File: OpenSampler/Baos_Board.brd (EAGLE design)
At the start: 57.2 x 26 mm, 33 parts, among them U1 FRAM, U2 DS3231ST&R

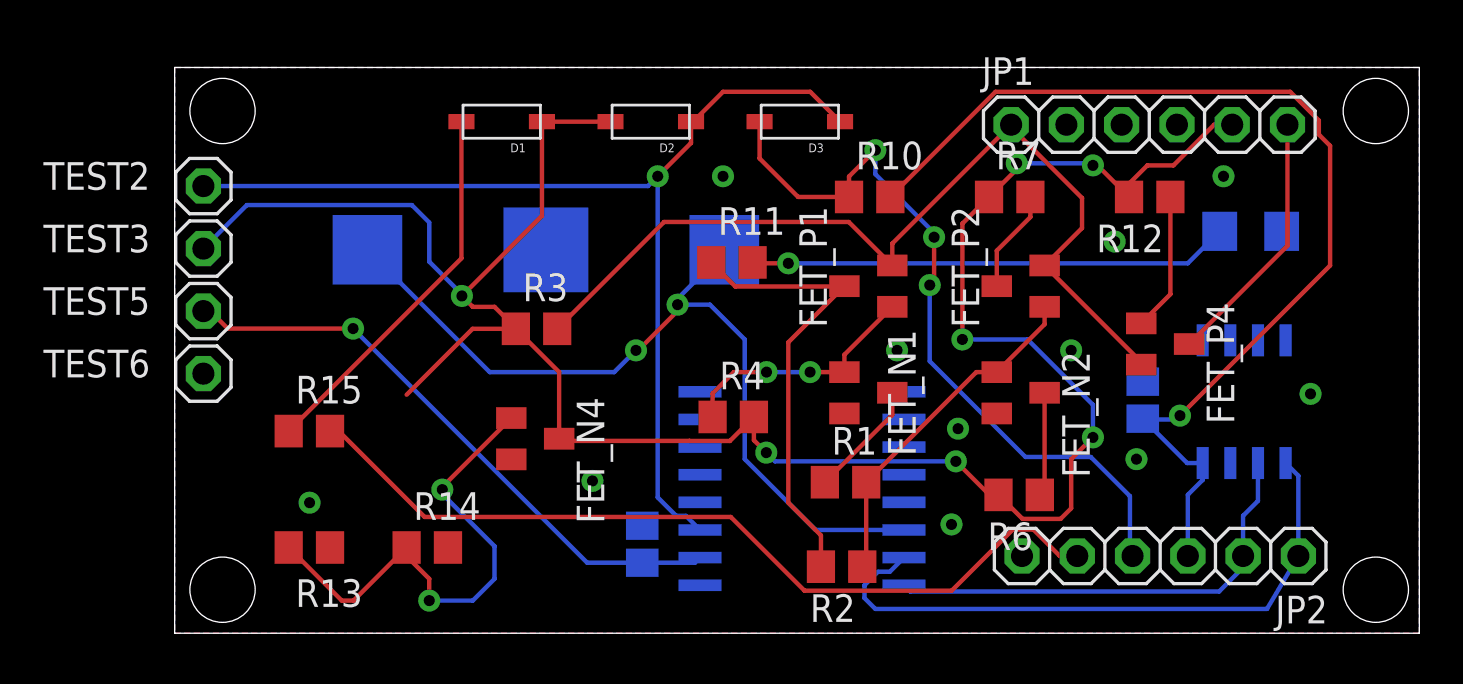
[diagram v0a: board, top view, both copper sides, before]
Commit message: Add files via upload
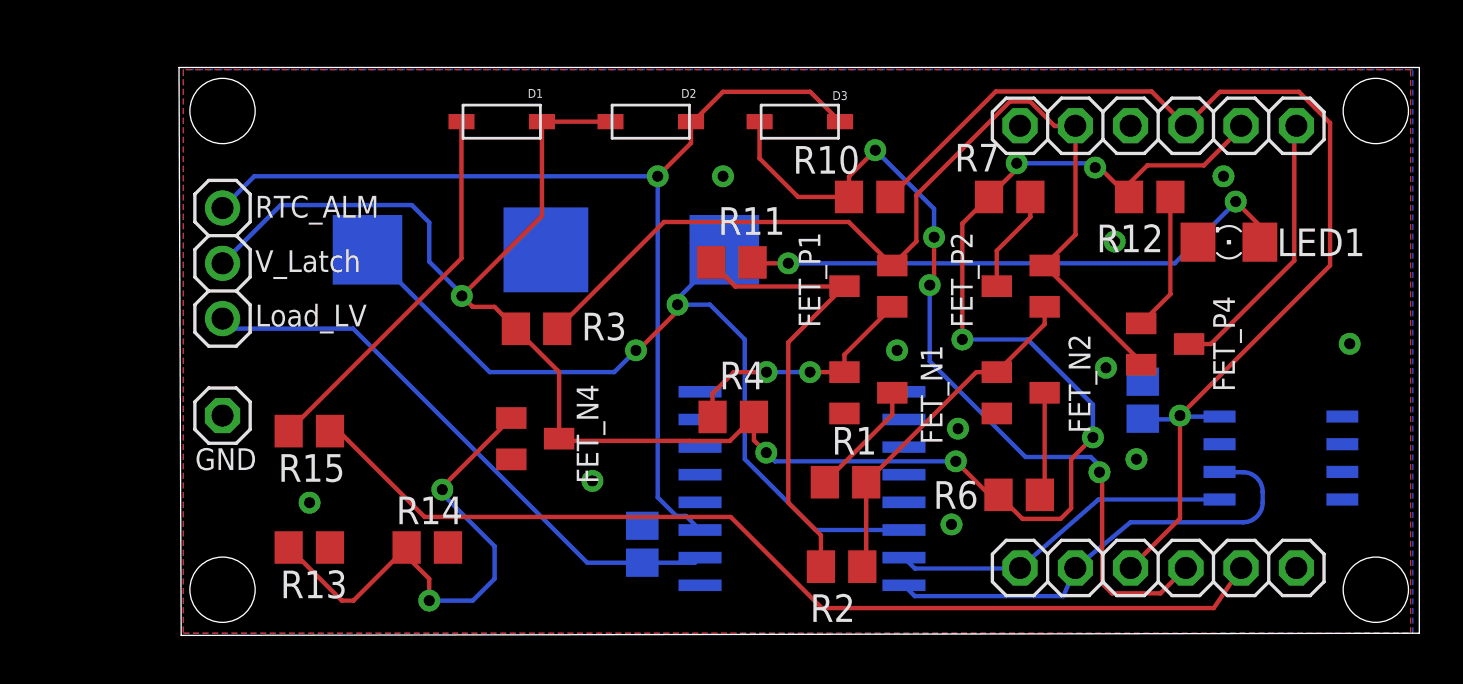
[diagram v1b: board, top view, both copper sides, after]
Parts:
- removed TEST2, TEST3, TEST5: (no value), pinhead:1X01
- removed U1: FRAM, power8:FPT-8P-M02
- added FRAM: FRAM, power8:FPT-8P-M02
- added JP3: (no value), adafruit:1X03
- R7: value 4.7k -> 500
- moved TEST6 2.12 mm to (-1.00, 10.0)
- moved LED1 1.12 mm to (45.2, 18.0), flipped to the top
- moved JP2 0.56 mm to (42.0, 3.00), turned to 0 degrees
- moved JP1 0.41 mm to (42.0, 23.3)
- renumbered U2 to RTC
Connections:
- net +12V: now also JP1.2; no longer JP1.1
- net +3V3: now also FRAM.8, JP1.4; no longer U1.8
- net GND: now also FRAM.4, JP1.1; no longer JP1.2, U1.4
- net LOAD_LV: now also JP3.3; no longer TEST5.1
- net RTC_ALM: now also JP3.1; no longer TEST2.1
- net SCL: now also FRAM.6; no longer U1.6
- net SDA: now also FRAM.5; no longer U1.5
- net V_LATCH: now also JP3.2; no longer TEST3.1
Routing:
- net SDA: track 29.0 -> 15.9 mm
- net SHDN: track 39.0 -> 46.2 mm
- net V_LATCH: track 104.1 -> 97.7 mm
- net ALM_READ: track 34.7 -> 39.9 mm, vias 3 -> 4
- net N$9: track 22.1 -> 25.7 mm, vias 1 -> 2
- net +3V3: track 48.8 -> 52.0 mm
- net +12V: track 41.9 -> 44.9 mm
- net LOAD_LV: track 27.7 -> 26.7 mm, vias 1 -> 0
- net REGULATOR: track 12.0 -> 12.7 mm
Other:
- board size 57.2 x 26 mm -> 57 x 26.1 mm
- board text added: "GND"
- board text added: "Load_LV"
- board text added: "RTC_ALM"
- board text added: "V_Latch"
